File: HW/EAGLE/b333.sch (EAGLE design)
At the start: 87 parts, among them Q5 NMOSD

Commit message: .
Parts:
- added 1C2: 220u/6V, resistor:CPOL-EUE3.5-8
- added 2C1: 0.47n, resistor:C-EUC0805K
- added 2D2: SS12, diode:SCHOTTKY-DIODESMD
- added 2L2: 220uH, rcl:L-US6000-XXX-RC
- added 2R5: 180R, resistor:R-EU_R0805
- added 2R6: 1R, resistor:R-EU_R0805
- added 2R7: 18K, resistor:R-EU_R0805
- added 2R8: 56K, resistor:R-EU_R0805
- added C4: 50u, resistor:CPOL-EUE2.5-6
- added C5, C6: 100n, resistor:C-EUC0805K
- added D7: MC34063AD, mc34063-2:MC34063AD
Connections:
- new net N$13: 2D2.A, 2L2.2, D7.SWC
- new net N$14: 2L2.1, 2R5.1, 2R6.2, D7.IS
- new net N$15: 2R5.2, D7.DC
- new net N$16: 2R7.2, 2R8.1, D7.FB
- new net N$8: 2C1.1, D7.TC
- net +5V: now also 1C2.+, 2D2.C, 2R8.2, C5.1
- net GND: now also 1C2.-, 2C1.2, 2R7.1, C4.-, C5.2, C6.2, D7.GND, D7.SWE
- net V+: now also 2R6.1, C4.+, C6.1, D7.VCC

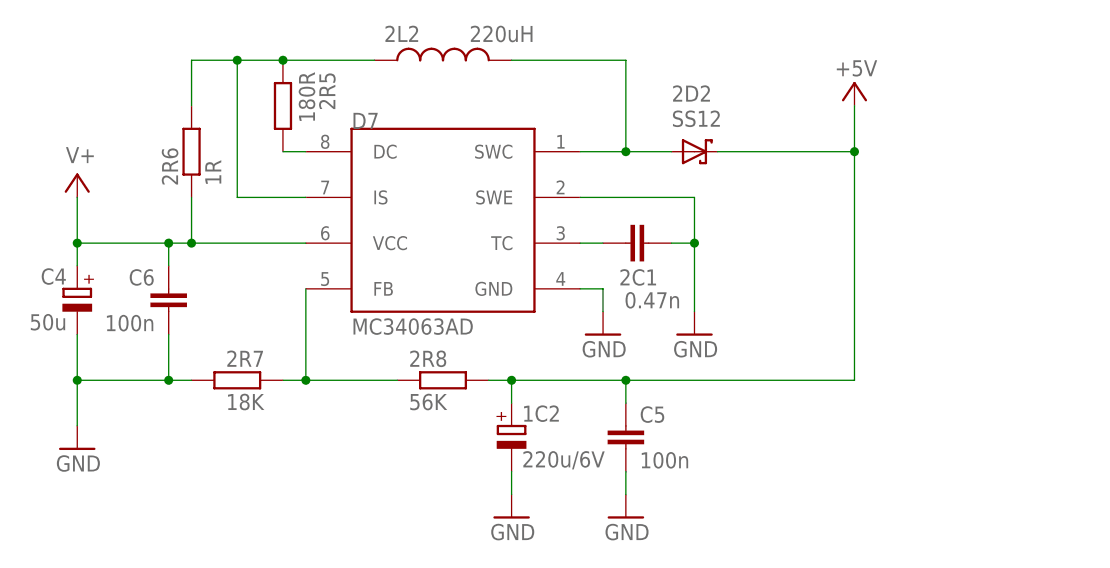
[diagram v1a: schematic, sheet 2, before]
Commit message: .
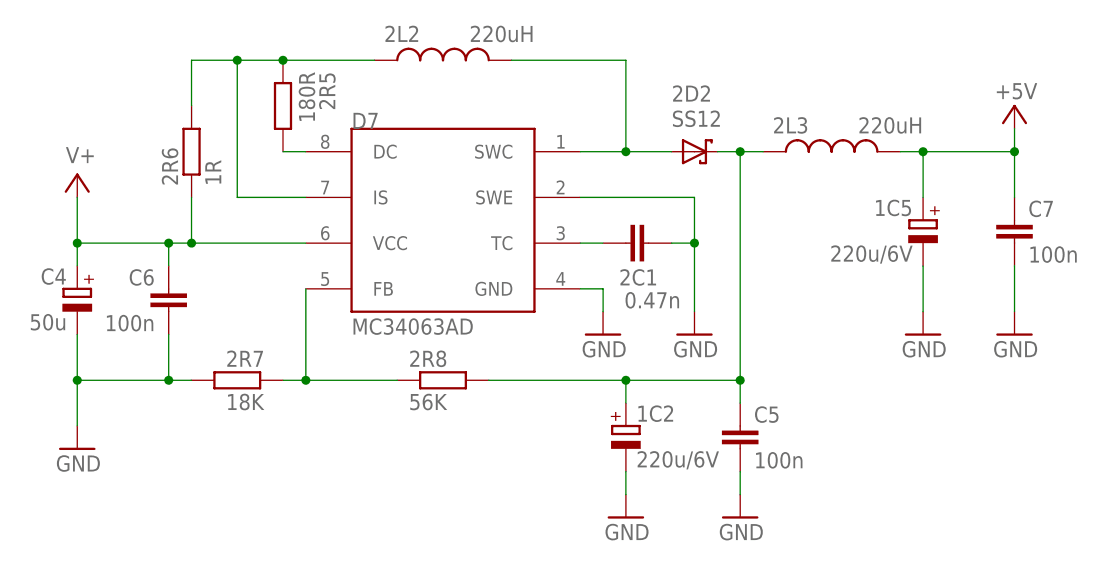
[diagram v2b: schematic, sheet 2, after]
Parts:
- added 1C5: 220u/6V, resistor:CPOL-EUE2-5
- added 2L3: 220uH, rcl:L-US6000-XXX-RC
- added C7: 100n, resistor:C-EUC0805K
- 1C2: device resistor:CPOL-EUE3.5-8 -> resistor:CPOL-EUE2-5
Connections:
- new net N$17: 1C2.+, 2D2.C, 2L3.1, 2R8.2, C5.1
- net +5V: now also 1C5.+, 2L3.2, C7.1; no longer 1C2.+, 2D2.C, 2R8.2, C5.1
- net GND: now also 1C5.-, C7.2
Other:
- moved on the sheet: 1C2, C5
